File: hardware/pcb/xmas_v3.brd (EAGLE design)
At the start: 160 x 100 mm, 53 parts, among them U1 ATTINY24-20SSU

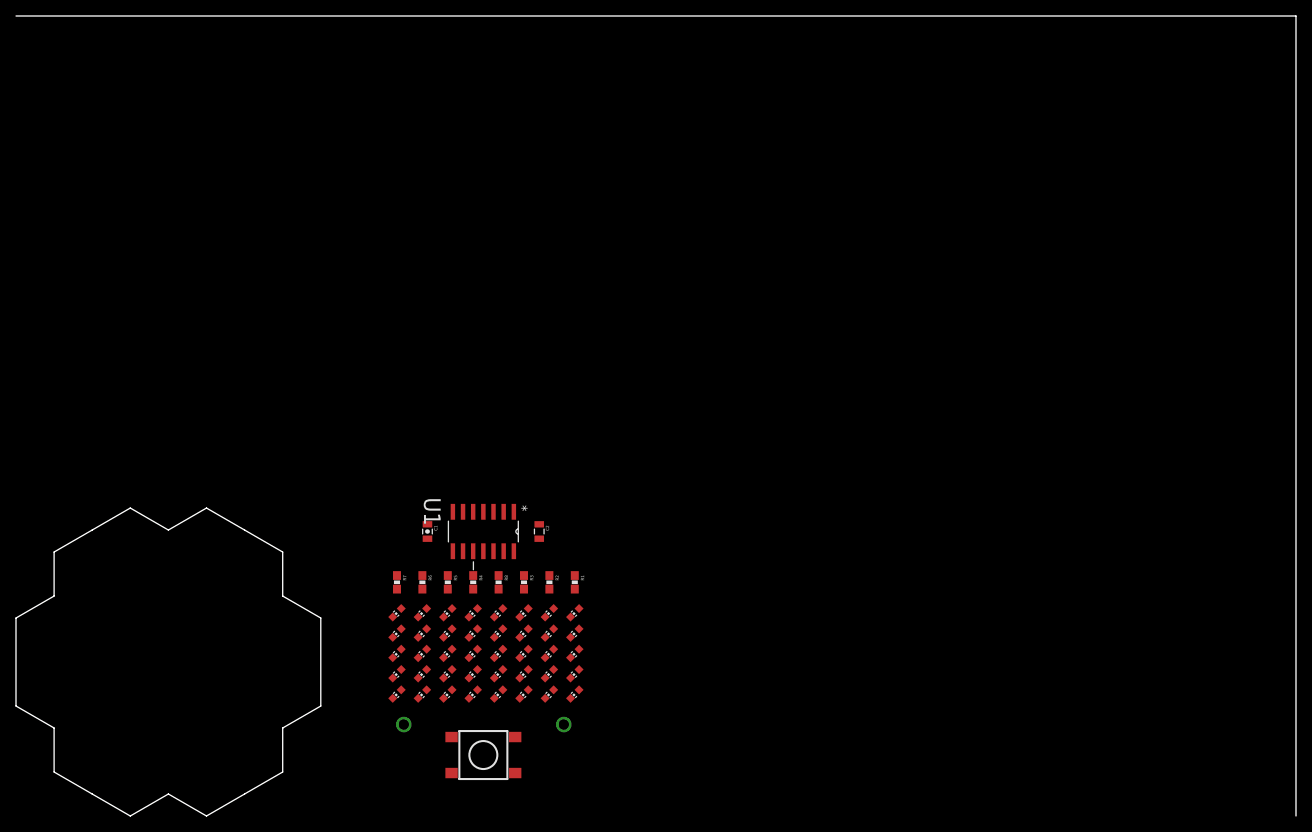
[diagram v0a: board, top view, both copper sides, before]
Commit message: Finished PCB design
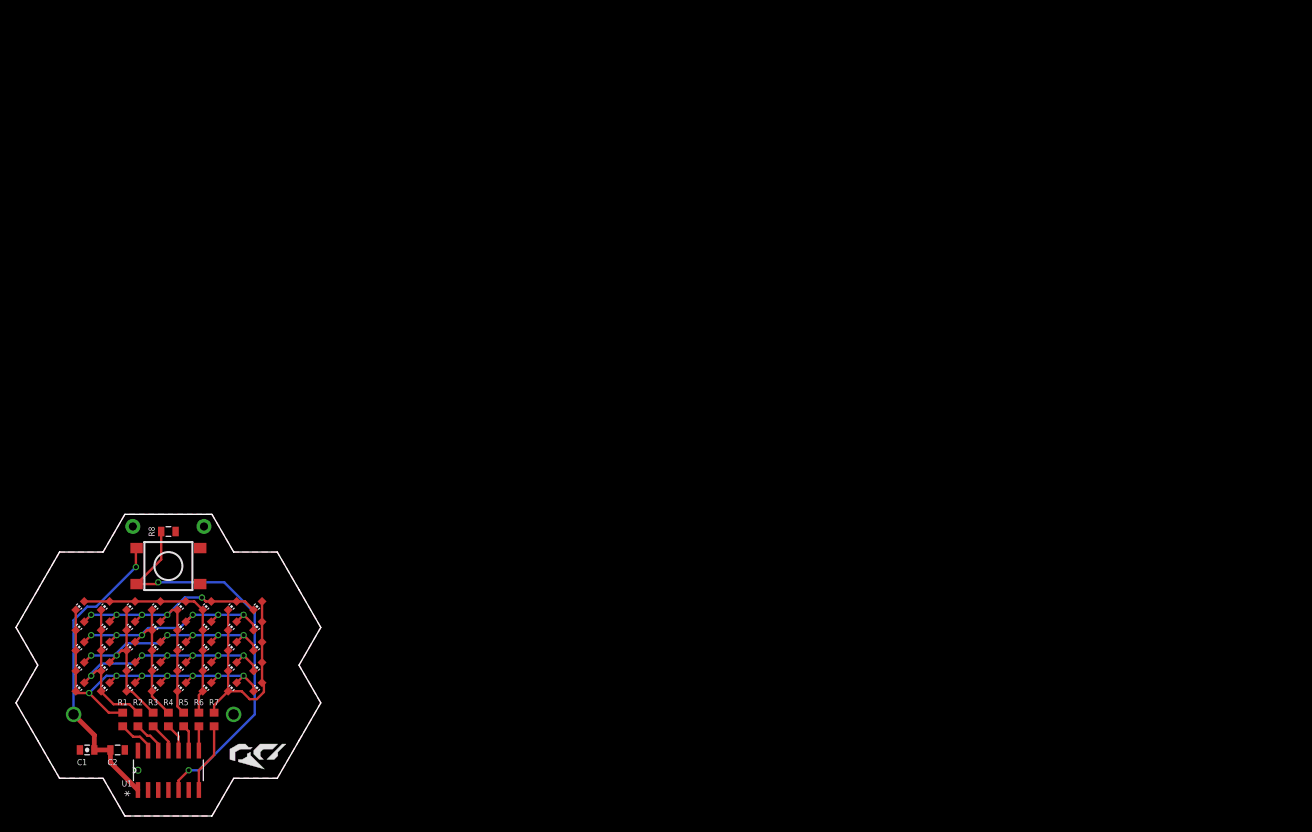
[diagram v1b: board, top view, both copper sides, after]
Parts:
- added JP1, JP2: (no value), SparkFun-Connectors:1X01_NO_SILK
- added U$1: (no value), ar1logo:AR1
- added U$2: (no value), ar1logo:XMAS
- R1, R2, R3, R4, R5, R6, R7: device SparkFun-Passives:0603-RES -> resistor:R0603
- R8: device SparkFun-Passives:0603-RES -> SparkFun-Passives:0805
- moved C2 59.4 mm to (12.7, 8.26), turned to 0 degrees
- moved R1 59.1 mm to (13.3, 12.1), turned to 90 degrees
- moved R2 54.2 mm to (15.2, 12.1), turned to 90 degrees
- moved C1 50.6 mm to (8.89, 8.26), turned to 180 degrees
- moved R3 49.4 mm to (17.1, 12.1), turned to 90 degrees
- moved U1 49.4 mm to (19.1, 5.71), turned to 90 degrees
- moved S1 45.9 mm to (19.1, 31.2), turned to 180 degrees
- moved R4 41.8 mm to (19.1, 12.1), turned to 90 degrees
- moved R8 41.8 mm to (19.1, 35.6), turned to 180 degrees
- moved BAT1 41.3 mm to (19.1, 12.7)
- moved D1 39.6 mm to (8.00, 16.1)
- moved D11 39.6 mm to (14.4, 16.1)
- moved D12 39.6 mm to (14.4, 18.7)
- moved D13 39.6 mm to (14.4, 21.2)
- moved D14 39.6 mm to (14.4, 23.7)
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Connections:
- net CA1: now also R1.2; no longer R7.2
- net CA2: now also R2.2; no longer R6.2
- net CA3: now also R3.2; no longer R5.2
- net CA5: now also R5.2; no longer R3.2
- net CA6: now also R6.2; no longer R2.2
- net CA7: now also R7.2; no longer R1.2
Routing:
- net N$2: track 0.00 -> 51.1 mm, vias 0 -> 2
- net CA2: track 0.00 -> 47.5 mm, vias 0 -> 6
- net CA1: track 0.00 -> 47.1 mm, vias 0 -> 7
- net CA3: track 0.00 -> 46.2 mm, vias 0 -> 6
- net CA4: track 0.00 -> 45.2 mm, vias 0 -> 6
- net CA5: track 0.00 -> 41.4 mm, vias 0 -> 5
- net N$1: track 0.00 -> 38.7 mm, vias 0 -> 1
- net CA7: track 0.00 -> 30.2 mm
- net CA6: track 0.00 -> 28.3 mm
- net N$9: track 0.00 -> 8.75 mm
- net N$3: track 0.00 -> 4.85 mm
- net N$4: track 0.00 -> 4.29 mm
- net N$5: track 0.00 -> 3.83 mm
- net N$6: track 0.00 -> 3.56 mm
- net N$7: track 0.00 -> 3.30 mm
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- added copper zone on layer 1, net GND
- added copper zone on layer 16, net GND
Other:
- board size 160 x 100 mm -> 38.1 x 37.7 mm
- board text added: "3V CR2032"
- board text added: "Merry Christmas from Blake"
- board text added: "Version 03 2016"
